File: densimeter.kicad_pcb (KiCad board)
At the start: 2 copper layers, 4 parts, among them IC1 XGZP6897A

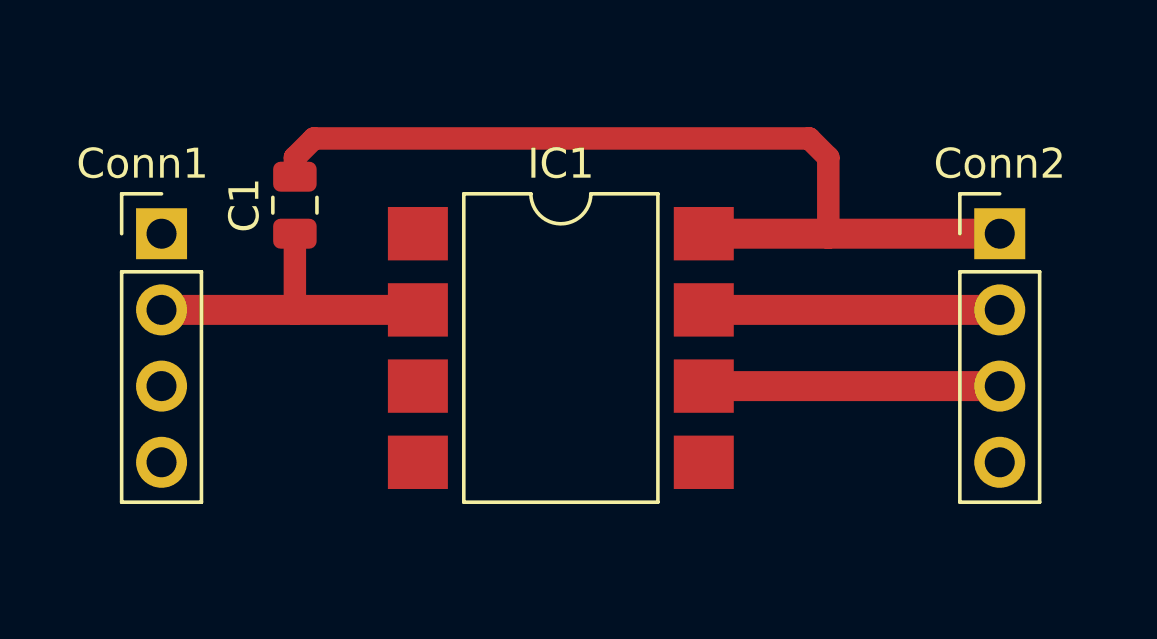
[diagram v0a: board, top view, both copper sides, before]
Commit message: 4 pins module
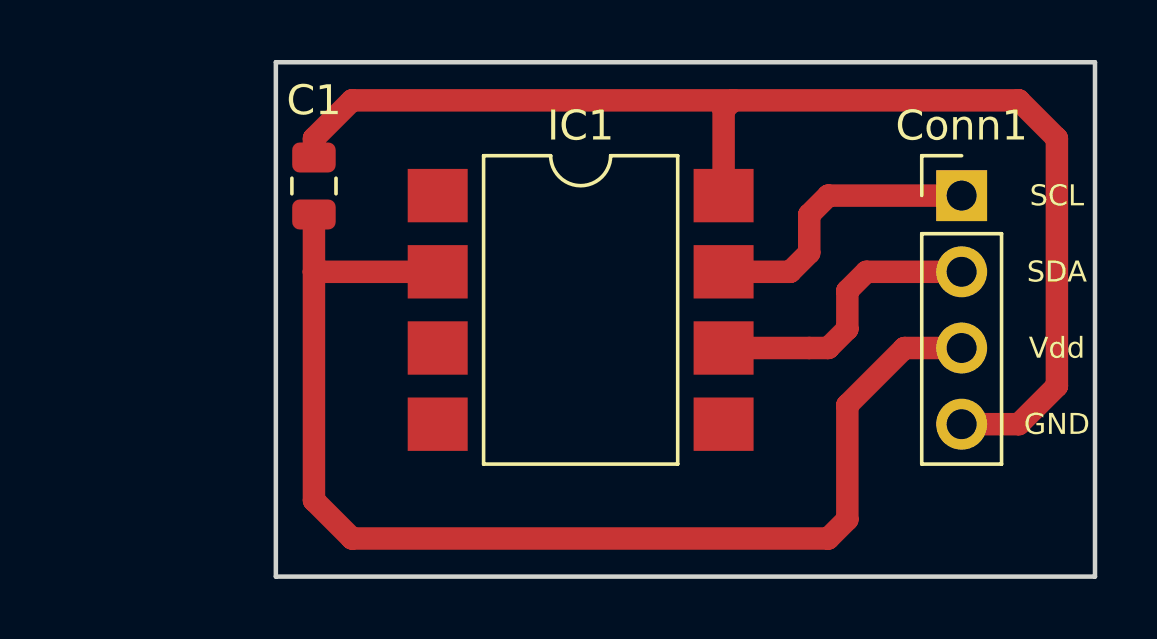
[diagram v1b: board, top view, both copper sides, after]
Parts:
- removed Conn2: CONN_4X1, Connector_PinHeader_2.54mm:PinHeader_1x04_P2.54mm_Vertical
- moved Conn1 26.7 mm to (25.4, 7.62)
- moved IC1 1.43 mm to (12.7, 11.4)
- moved C1 0.90 mm to (3.81, 7.30)
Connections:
- C1 pad 2: /GND -> /Gnd
- Conn1 pad 1: (no net) -> /SCL
- Conn1 pad 2: /Vdd -> /SDA
- Conn1 pad 3: (no net) -> /Vdd
- Conn1 pad 4: (no net) -> /Gnd
- IC1 pad 8: /GND -> /Gnd
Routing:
- net /Gnd: track 0.00 -> 41.7 mm
- net /Vdd: track 10.1 -> 40.6 mm
- net /GND: track 30.4 -> 0.00 mm
- net /SDA: track 8.89 -> 9.73 mm
- net /SCL: track 8.89 -> 9.73 mm
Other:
- board outline added: 27.3 x 17.1 mm
- board text added: "GND"
- board text added: "SCL"
- board text added: "SDA"
- board text added: "Vdd"
